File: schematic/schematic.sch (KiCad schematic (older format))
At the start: 15 parts, among them Q1 IRLZ34N, SW1 MODE, SW2 UP, SW3 DOWN, SW4 SW_Push, U1 TM1637Display

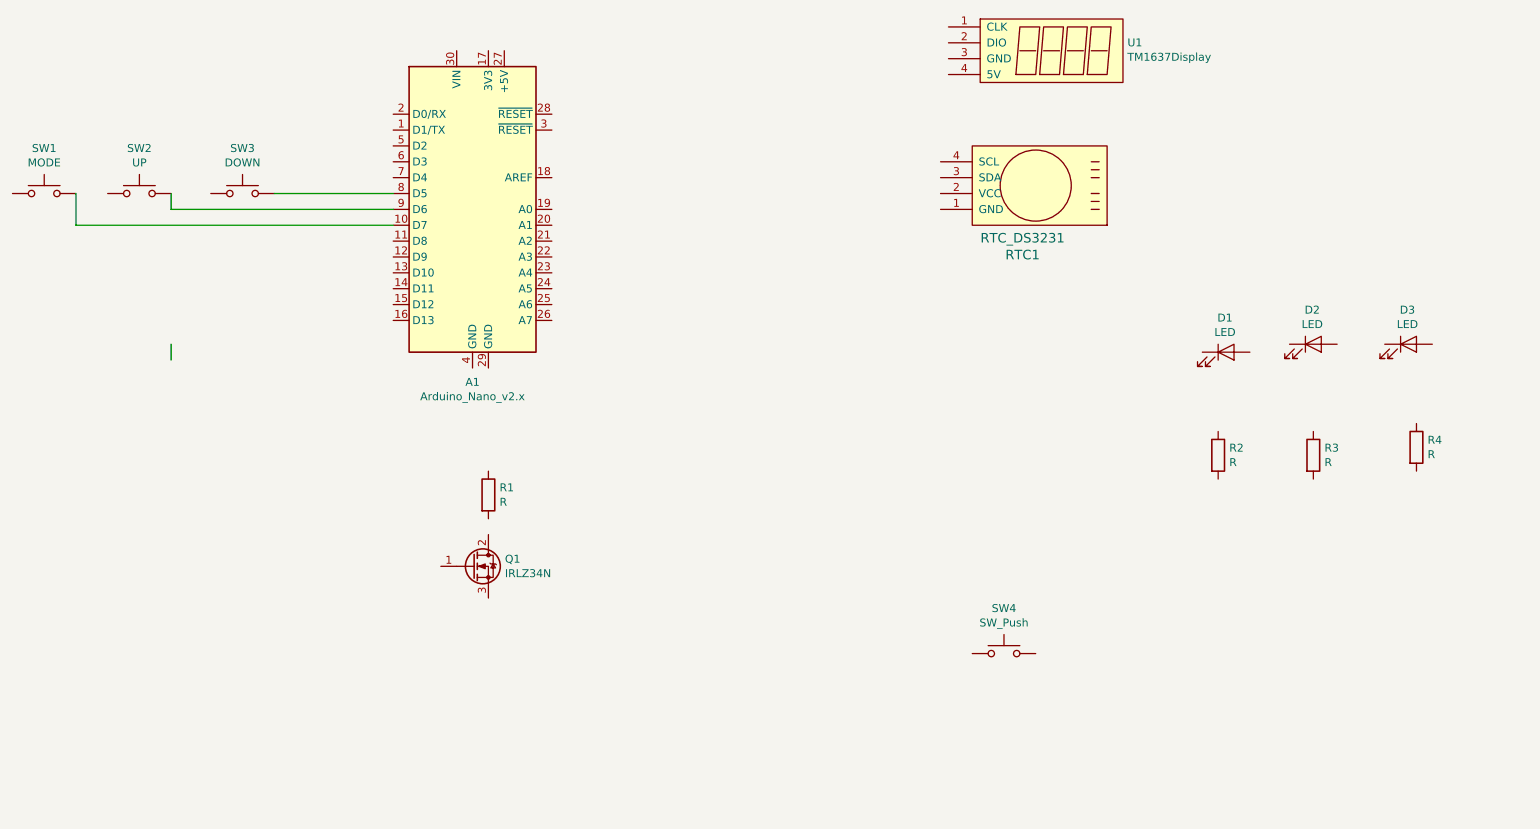
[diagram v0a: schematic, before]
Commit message: draw schematics
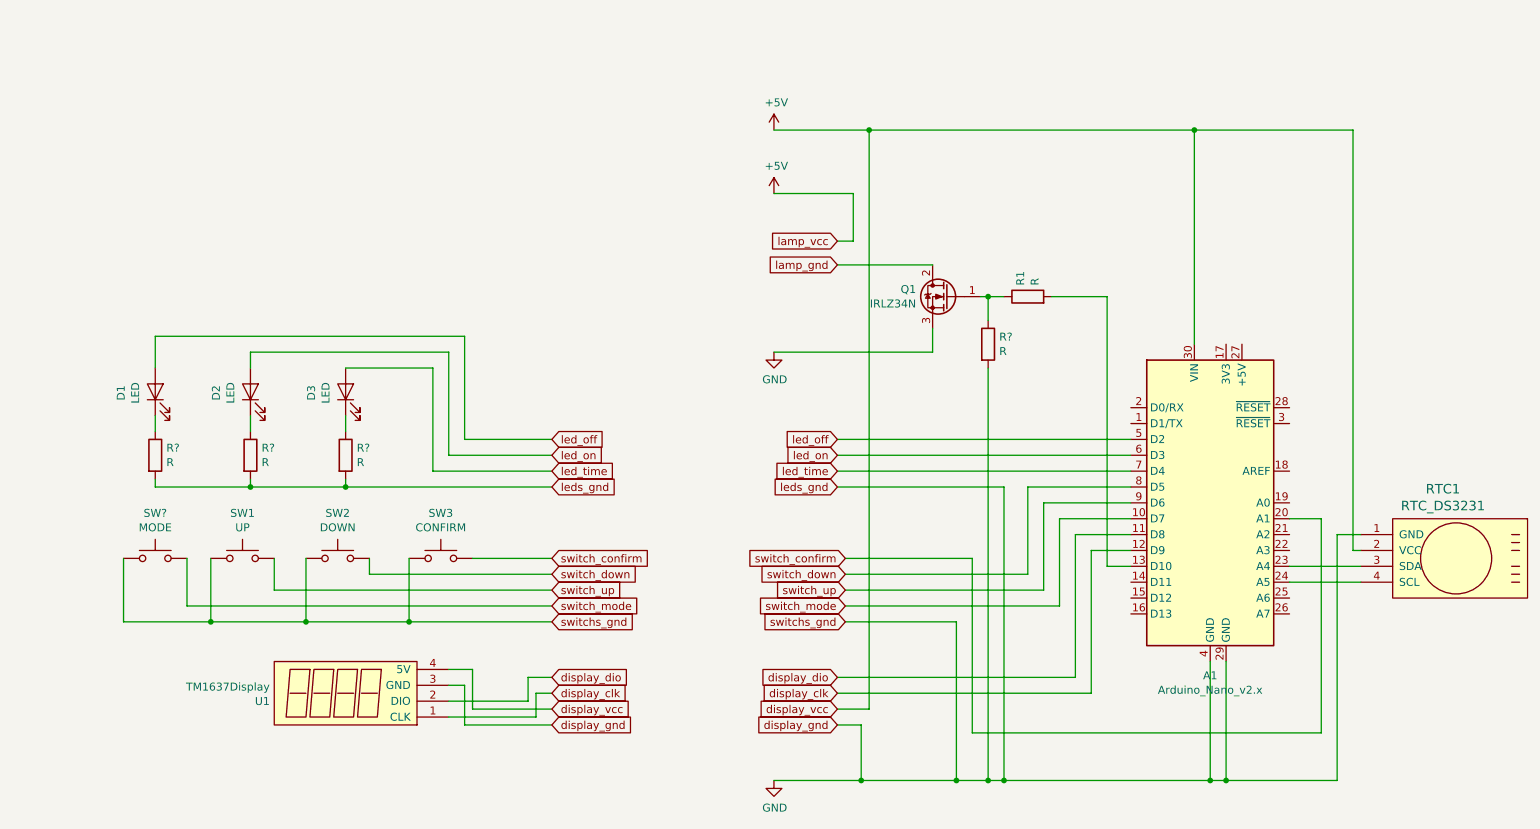
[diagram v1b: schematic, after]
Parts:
- removed R2, R3, R4: R, Resistor_THT:R_Axial_DIN0204_L3.6mm_D1.6mm_P5.08mm_Vertical, symbol Device:R
- removed SW4: SW_Push, Button_Switch_THT:SW_PUSH_6mm_H5mm, symbol Switch:SW_Push
- added R? (x4): R, Resistor_THT:R_Axial_DIN0204_L3.6mm_D1.6mm_P5.08mm_Vertical, symbol Device:R
- added SW?: MODE, Button_Switch_THT:SW_PUSH_6mm_H5mm, symbol Switch:SW_Push
- SW1: value MODE -> UP
- SW2: value UP -> DOWN
- SW3: value DOWN -> CONFIRM
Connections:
- net labels added: +5V, GND, display_clk, display_dio, display_gnd, display_vcc, lamp_gnd, lamp_vcc, led_off, led_on, led_time, leds_gnd, switch_confirm, switch_down, switch_mode, switch_up, switchs_gnd
- wire segments 6 -> 110
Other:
- moved on the sheet: A1, D1, D2, D3, Q1, R1, RTC1, SW1, SW2, SW3, U1
